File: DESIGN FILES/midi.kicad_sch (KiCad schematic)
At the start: 7 parts

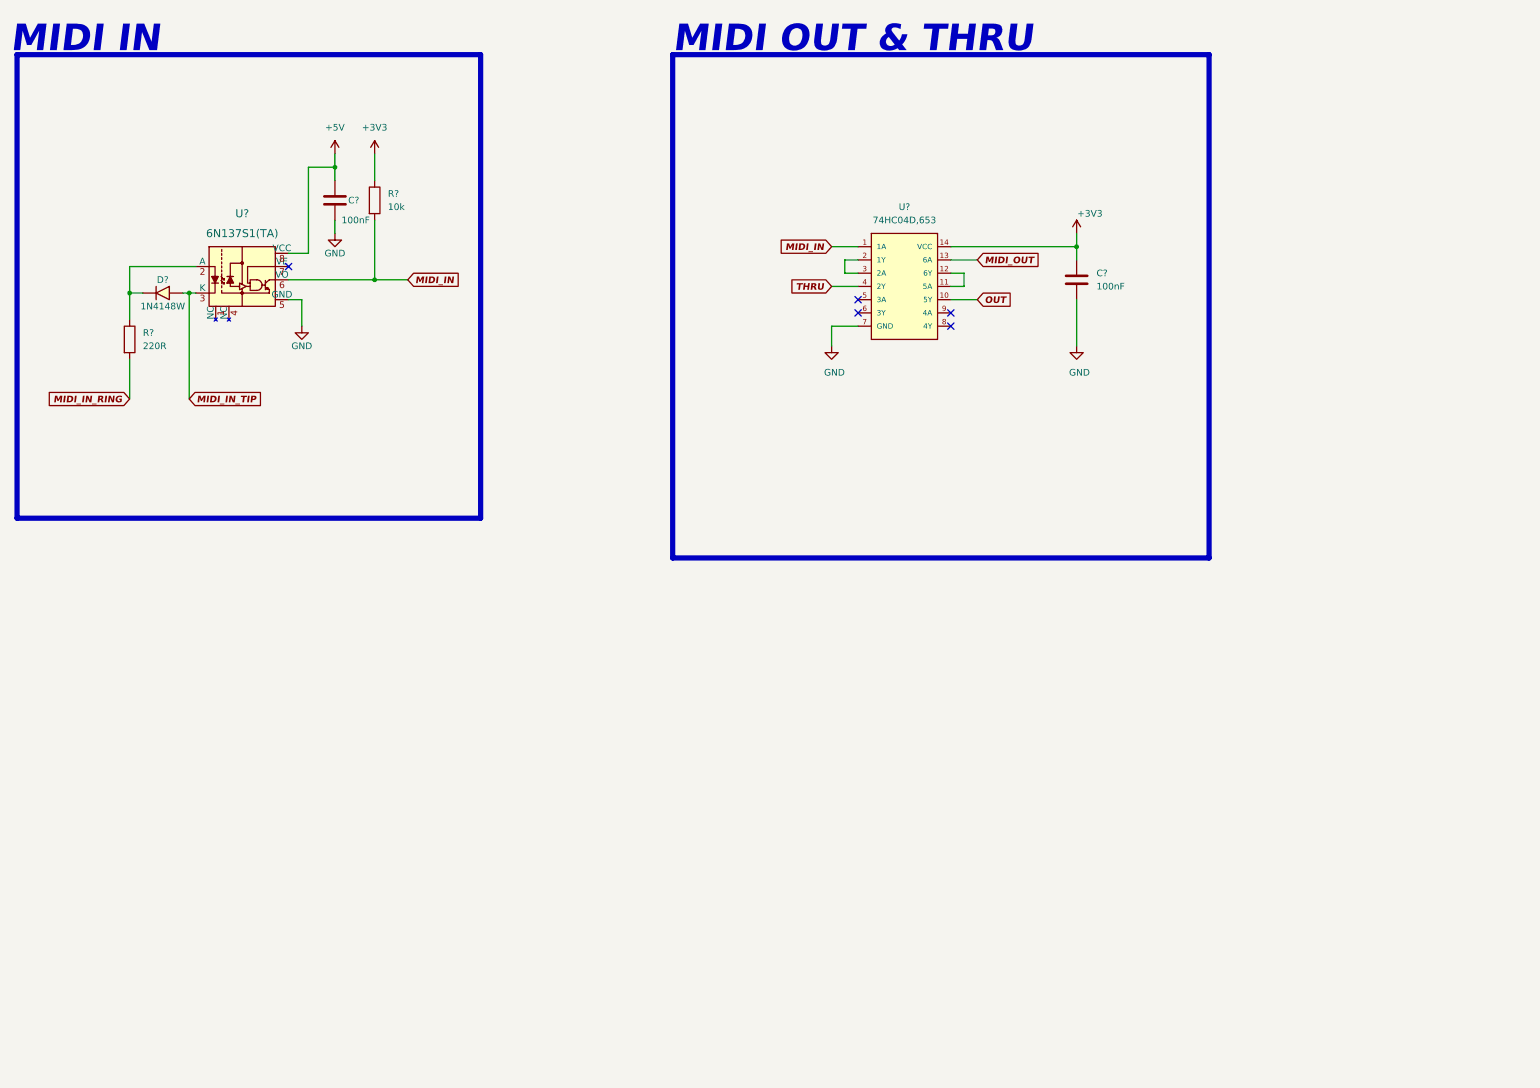
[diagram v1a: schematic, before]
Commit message: updates
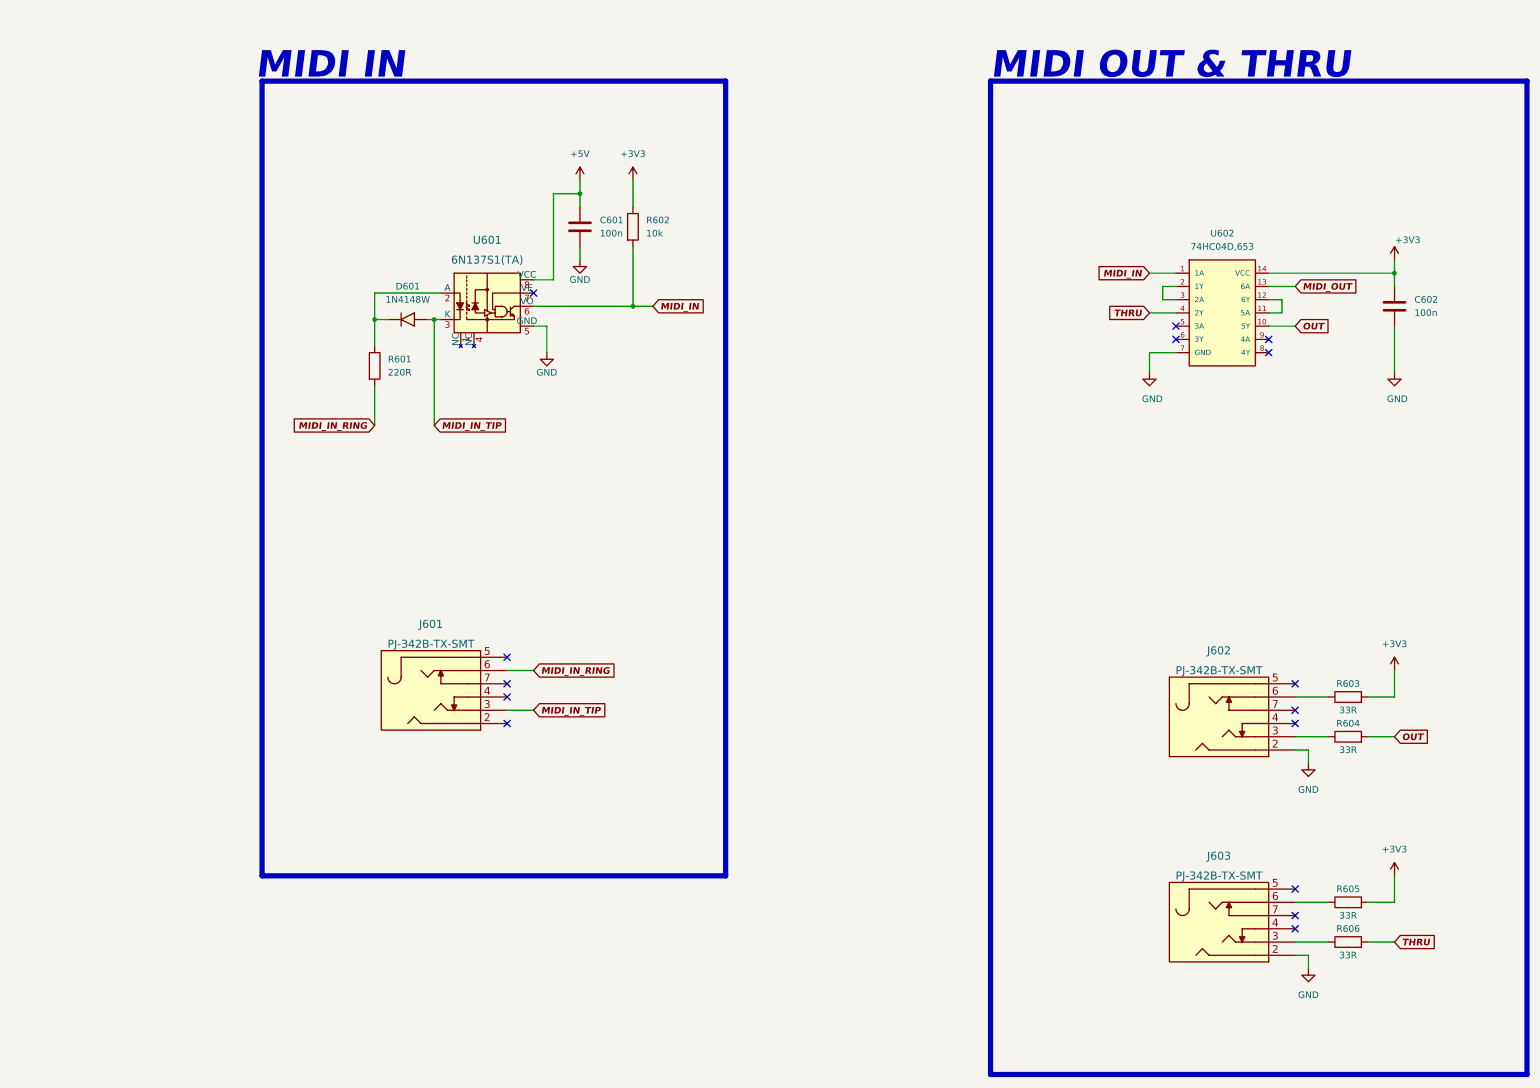
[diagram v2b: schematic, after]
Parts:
- removed C? (x2): 100nF, soundsom:CC0603KRX7R9BB104_0603, symbol soundsom:CC0603KRX7R9BB104
- removed D?: 1N4148W, soundsom:1N4148W_SOD-123, symbol soundsom:1N4148W
- removed R?: 220R, soundsom:0603WAF2200T5E_0603, symbol soundsom:0603WAF2200T5E
- removed R?: 10k, soundsom:0603WAF1002T5E_0603, symbol soundsom:0603WAF1002T5E
- removed U?: 6N137S1(TA), soundsom:6N137S1_TA_SMD-8P, symbol soundsom:6N137S1(TA)
- removed U?: 74HC04D,653, soundsom:74HC04D_653_SOIC-14, symbol soundsom:74HC04D,653
- added C601, C602: 100n, MY CAPACITOR LIBRARY:CC0603KRX7R9BB104_0603, symbol MY CAPACITOR LIBRARY:CC0603KRX7R9BB104
- added D601: 1N4148W, MY DIODE LIBRARY:1N4148W_SOD-123, symbol MY DIODE LIBRARY:1N4148W
- added J601, J602, J603: PJ-342B-TX-SMT, MY CONNECTOR LIBRARY:PJ-342B-TX-SMT, symbol MY CONNECTOR LIBRARY:PJ-342B-TX-SMT
- added R601: 220R, MY RESISTOR LIBRARY:0603WAF2200T5E, symbol MY RESISTOR LIBRARY:0603WAF2200T5E
- added R602: 10k, MY RESISTOR LIBRARY:0603WAF1002T5E, symbol MY RESISTOR LIBRARY:0603WAF1002T5E
- added R603, R604, R605, R606: 33R, MY RESISTOR LIBRARY:0805W8F330JT5E, symbol MY RESISTOR LIBRARY:0603WAF330JT5E
- added U601: 6N137S1(TA), MY OPTO IC LIBRARY:6N137S1_TA_SMD-8P, symbol MY OPTO IC LIBRARY:6N137S1(TA)
- added U602: 74HC04D,653, MY IC LIBRARY:74HC04D_653_SOIC-14, symbol MY IC LIBRARY:74HC04D,653
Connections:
- net +3V3: now also C602.1, R602.1, R603.2, R605.2, U602.14 (VCC)
- net +5V: now also C601.1, U601.8 (VCC)
- net GND: now also C601.2, C602.2, J602.2, J603.2, U601.5 (GND), U602.7 (GND)
- net MIDI_IN: now also R602.2, U601.6 (VO), U602.1 (1A)
- net MIDI_IN_RING: now also J601.6, R601.2
- net MIDI_IN_TIP: now also D601.2 (A), J601.3, U601.3 (K)
- net MIDI_OUT: now also U602.13 (6A)
- net OUT: now also R604.2, U602.10 (5Y)
- net THRU: now also R606.2, U602.4 (2Y)
- new net: J603.3, R606.1
- new net: J603.6, R605.1
- new net: D601.1 (K), R601.1, U601.2 (A)
- new net: U602.11 (5A), U602.12 (6Y)
- new net: U602.2 (1Y), U602.3 (2A)
- new net: J602.6, R603.1
- new net: J602.3, R604.1
- no-connect marks 5 -> 15
